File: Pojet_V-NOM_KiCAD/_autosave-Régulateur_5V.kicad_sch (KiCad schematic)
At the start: 15 parts, among them IC2 MP1475SGJ-P

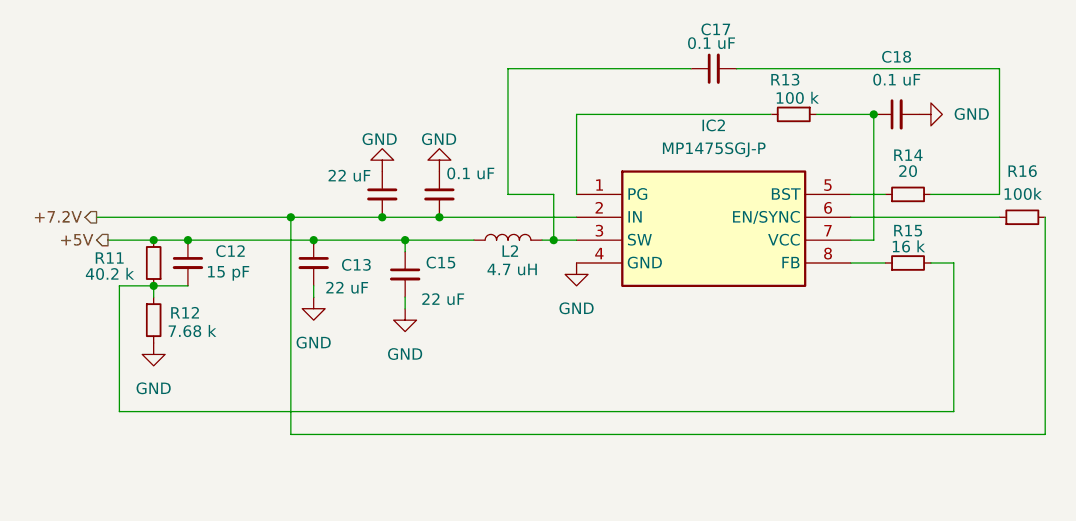
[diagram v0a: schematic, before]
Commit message: modif
modif
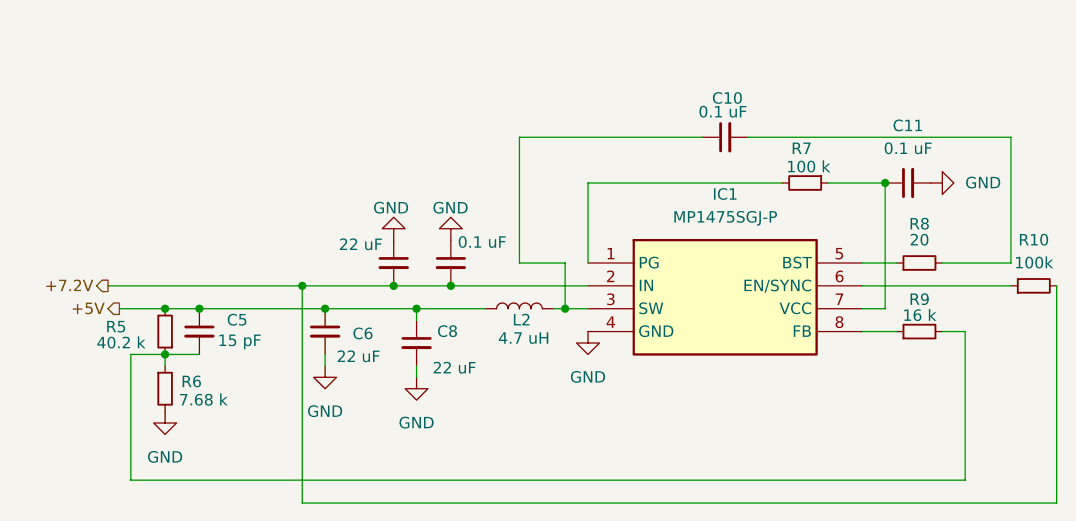
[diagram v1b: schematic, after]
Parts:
- removed C12: 15 pF, symbol Device:C_Small
- removed C13, C14, C15: 22 uF, symbol Device:C_Small
- removed C16, C17, C18: 0.1 uF, symbol Device:C_Small
- removed IC2: MP1475SGJ-P, SOT65P280X100-8N, symbol MP1475SGJ-P:MP1475SGJ-P
- removed R11: 40.2 k, symbol Device:R_Small
- removed R12: 7.68 k, symbol Device:R_Small
- removed R13: 100 k, symbol Device:R_Small
- removed R14: 20, symbol Device:R_Small
- removed R15: 16 k, symbol Device:R_Small
- removed R16: 100k, symbol Device:R_Small
- added C10, C11, C9: 0.1 uF, symbol Device:C_Small
- added C5: 15 pF, symbol Device:C_Small
- added C6, C7, C8: 22 uF, symbol Device:C_Small
- added IC1: MP1475SGJ-P, SOT65P280X100-8N, symbol MP1475SGJ-P:MP1475SGJ-P
- added R10: 100k, symbol Device:R_Small
- added R5: 40.2 k, symbol Device:R_Small
- added R6: 7.68 k, symbol Device:R_Small
- added R7: 100 k, symbol Device:R_Small
- added R8: 20, symbol Device:R_Small
- added R9: 16 k, symbol Device:R_Small
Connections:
- net +5V: now also C5.1, C6.1, C8.1, R5.2
- net +7.2V: now also C7.2, C9.2, IC1.2 (IN), R10.2
- net GND: now also C11.2, C6.2, C7.1, C8.2, C9.1, IC1.4 (GND), R6.2
- net at L2.2: now also C10.1, IC1.3 (SW)
- new net: C10.2, R8.2
- new net: IC1.6 (EN/SYNC), R10.1
- new net: C5.2, R5.1, R6.1, R9.2
- new net: IC1.8 (FB), R9.1
- new net: C11.1, IC1.7 (VCC), R7.1
- new net: IC1.1 (PG), R7.2
- new net: IC1.5 (BST), R8.1
